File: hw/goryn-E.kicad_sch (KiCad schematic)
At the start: 11 parts, among them J3 Conn_FFC_30, U2 W25Q128JVS

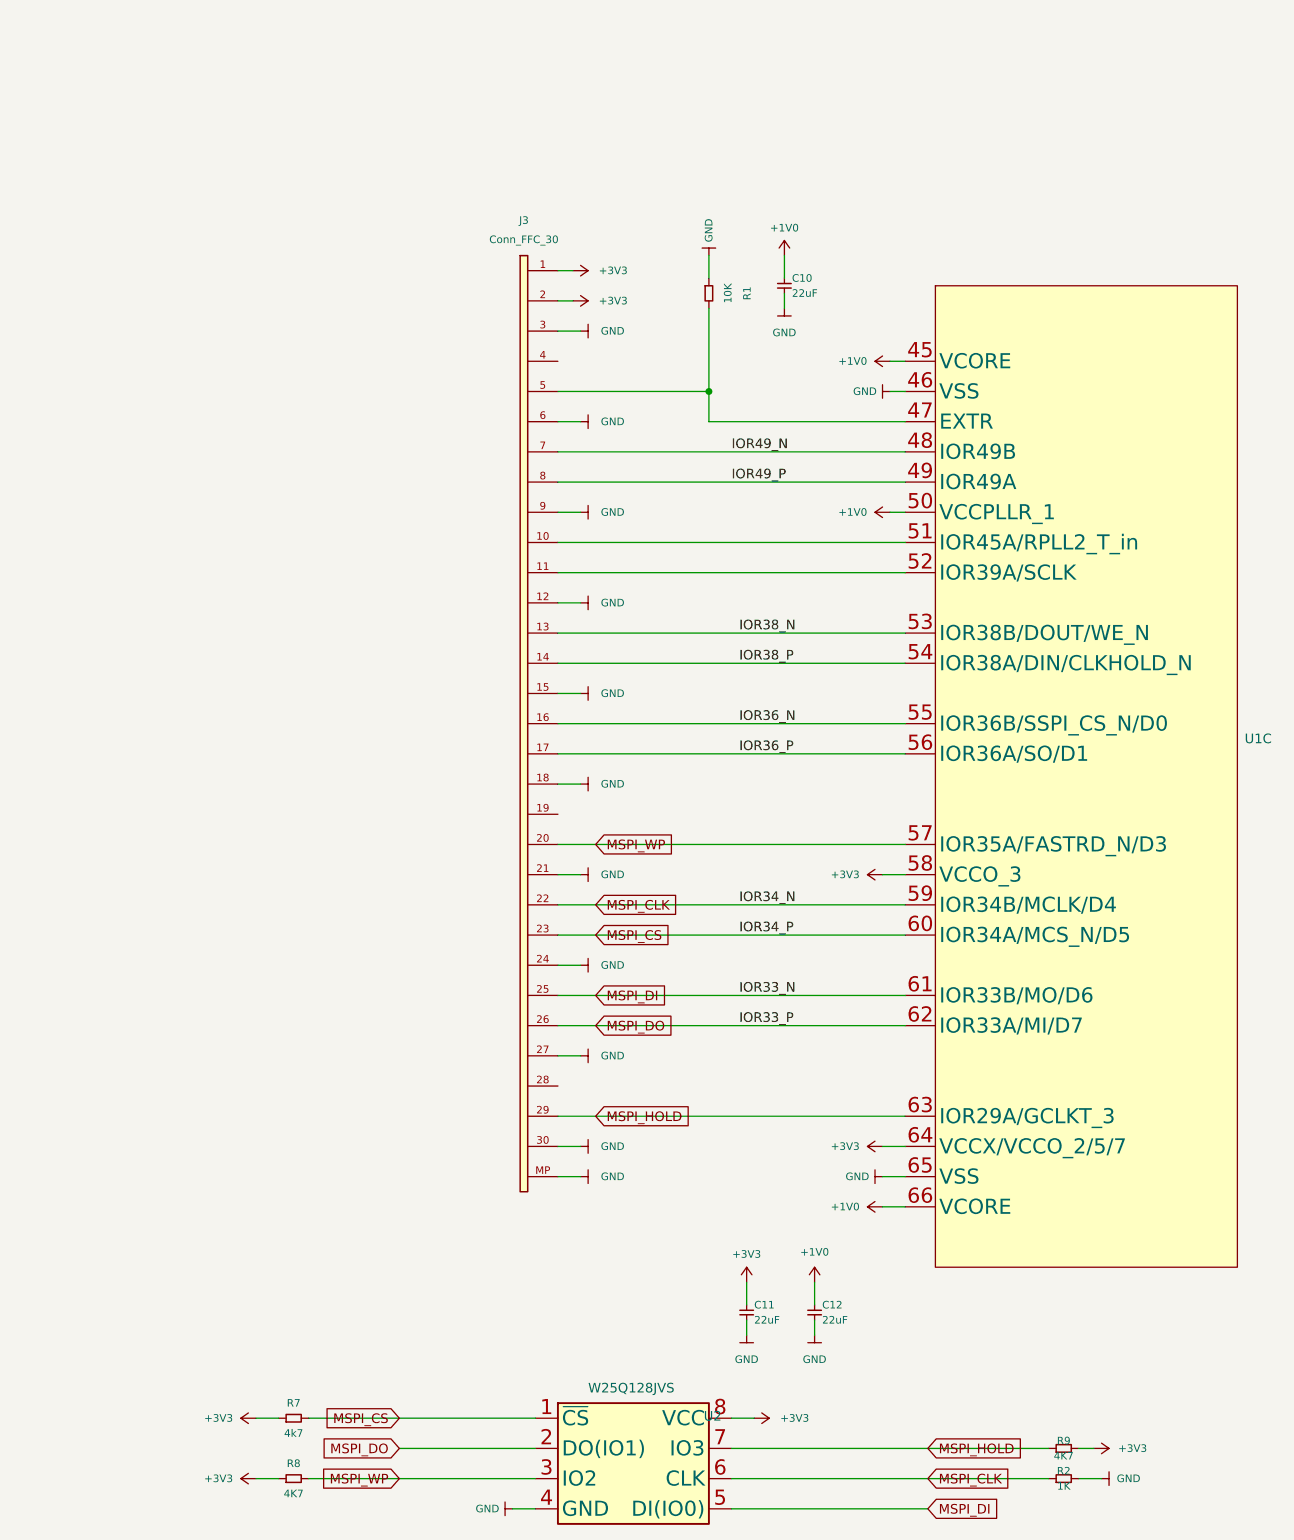
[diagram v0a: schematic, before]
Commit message: happy kicad 8
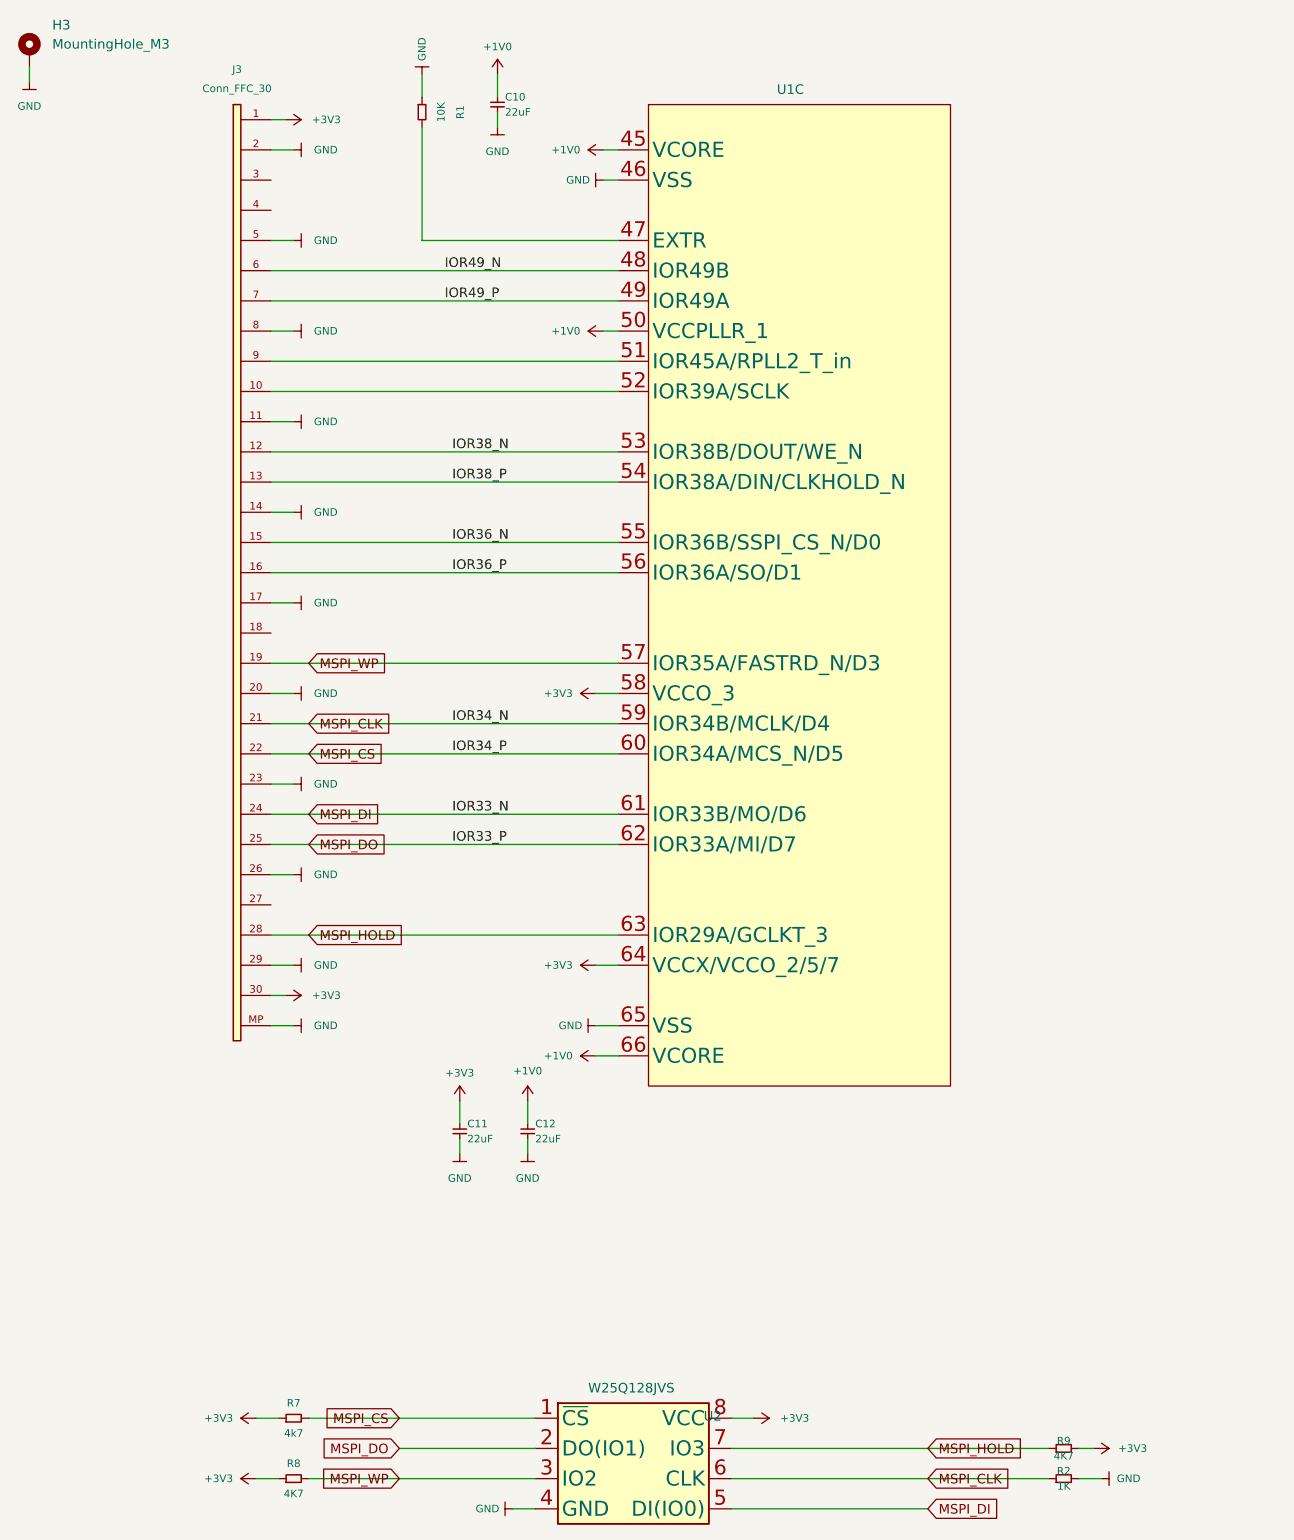
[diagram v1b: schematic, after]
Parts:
- added H3: MountingHole_M3, AI6YP:MountingHole_3.2mm_M3_Pad_Via, symbol AI6YP:MountingHole_M3
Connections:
- net +3V3: now also J3.30 (Pin_30); no longer J3.2 (Pin_2)
- net GND: now also J3.11 (Pin_11), J3.14 (Pin_14), J3.17 (Pin_17), J3.2 (Pin_2), J3.20 (Pin_20), J3.23 (Pin_23), J3.26 (Pin_26), J3.29 (Pin_29), J3.5 (Pin_5), J3.8 (Pin_8), H3.1; no longer J3.12 (Pin_12), J3.15 (Pin_15), J3.18 (Pin_18), J3.21 (Pin_21), J3.24 (Pin_24), J3.27 (Pin_27), J3.3 (Pin_3), J3.30 (Pin_30), J3.6 (Pin_6), J3.9 (Pin_9)
- net IOR36_N: now also J3.15 (Pin_15); no longer J3.16 (Pin_16)
- net IOR36_P: now also J3.16 (Pin_16); no longer J3.17 (Pin_17)
- net IOR38_N: now also J3.12 (Pin_12); no longer J3.13 (Pin_13)
- net IOR38_P: now also J3.13 (Pin_13); no longer J3.14 (Pin_14)
- net IOR49_N: now also J3.6 (Pin_6); no longer J3.7 (Pin_7)
- net IOR49_P: now also J3.7 (Pin_7); no longer J3.8 (Pin_8)
- net MSPI_CLK: now also J3.21 (Pin_21); no longer J3.22 (Pin_22)
- net MSPI_CS: now also J3.22 (Pin_22); no longer J3.23 (Pin_23)
- net MSPI_DI: now also J3.24 (Pin_24); no longer J3.25 (Pin_25)
- net MSPI_DO: now also J3.25 (Pin_25); no longer J3.26 (Pin_26)
- net MSPI_HOLD: now also J3.28 (Pin_28); no longer J3.29 (Pin_29)
- net MSPI_WP: now also J3.19 (Pin_19); no longer J3.20 (Pin_20)
- net at J3.10 (Pin_10): now also U1.52 (IOR39A/SCLK); no longer U1.51 (IOR45A/RPLL2_T_in)
- net at R1.2, U1.47 (EXTR): no longer J3.5 (Pin_5)
- new net: J3.9 (Pin_9), U1.51 (IOR45A/RPLL2_T_in)
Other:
- moved on the sheet: C10, C11, C12, J3, R1, U1C
